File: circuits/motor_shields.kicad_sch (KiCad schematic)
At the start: 24 parts, among them IC1 BTN70301EPAXUMA1, IC2 BTN70301EPAXUMA1, IC3 BTN70301EPAXUMA1, IC4 BTN70301EPAXUMA1, J4 Conn_01x02_Pin, U2 74HC244

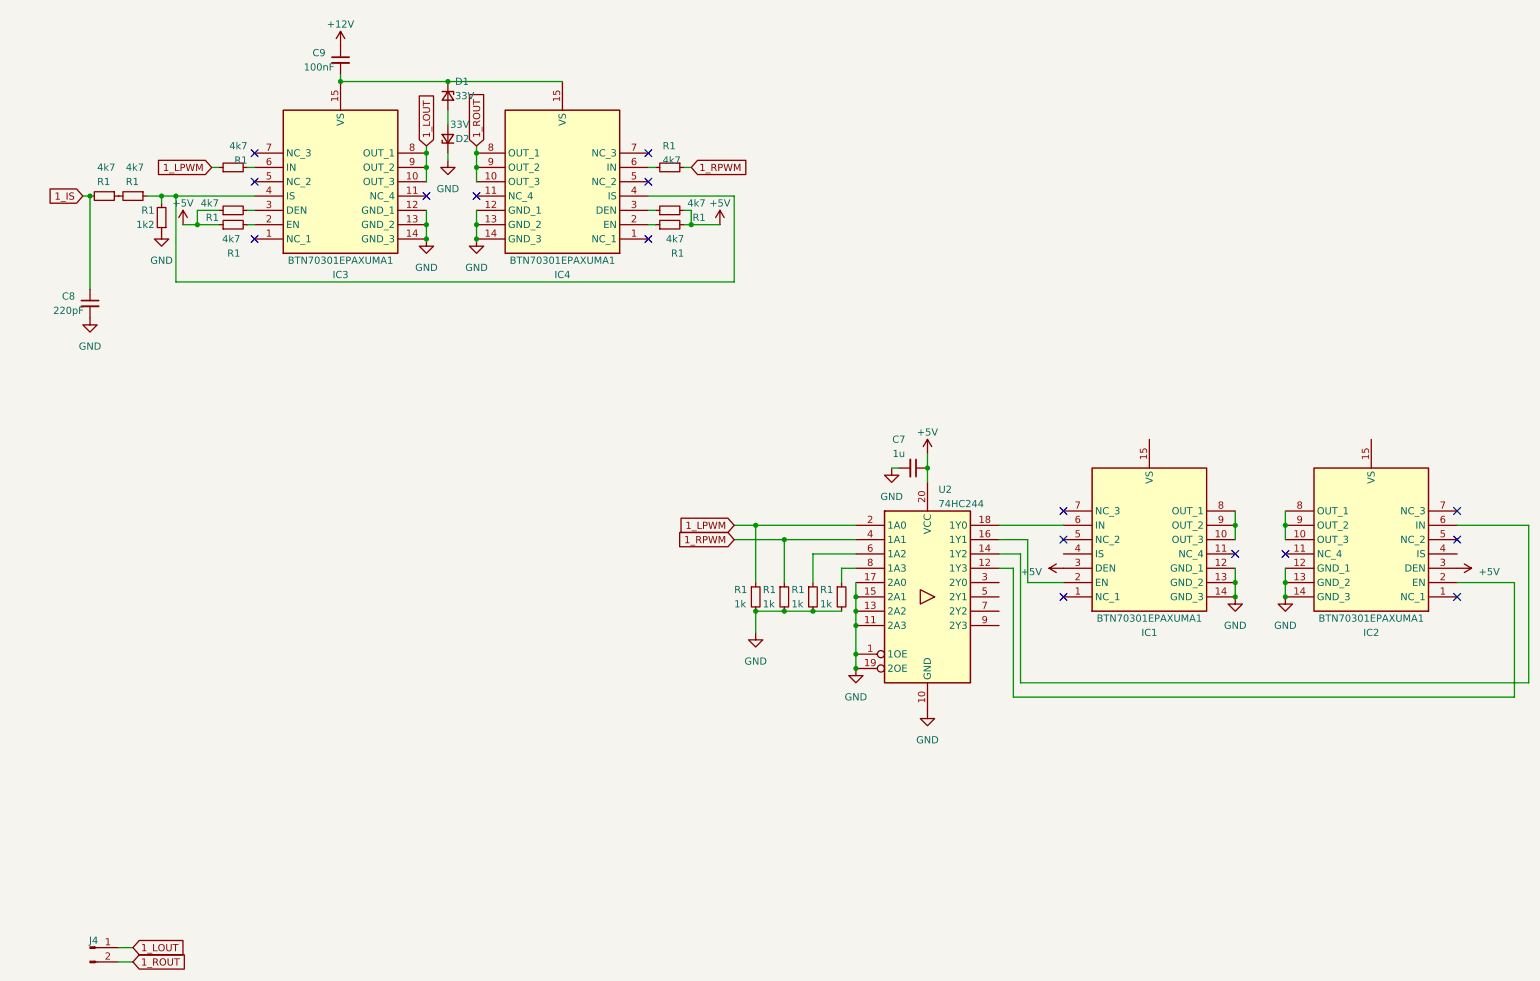
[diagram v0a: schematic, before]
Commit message: controller pcb rev 1
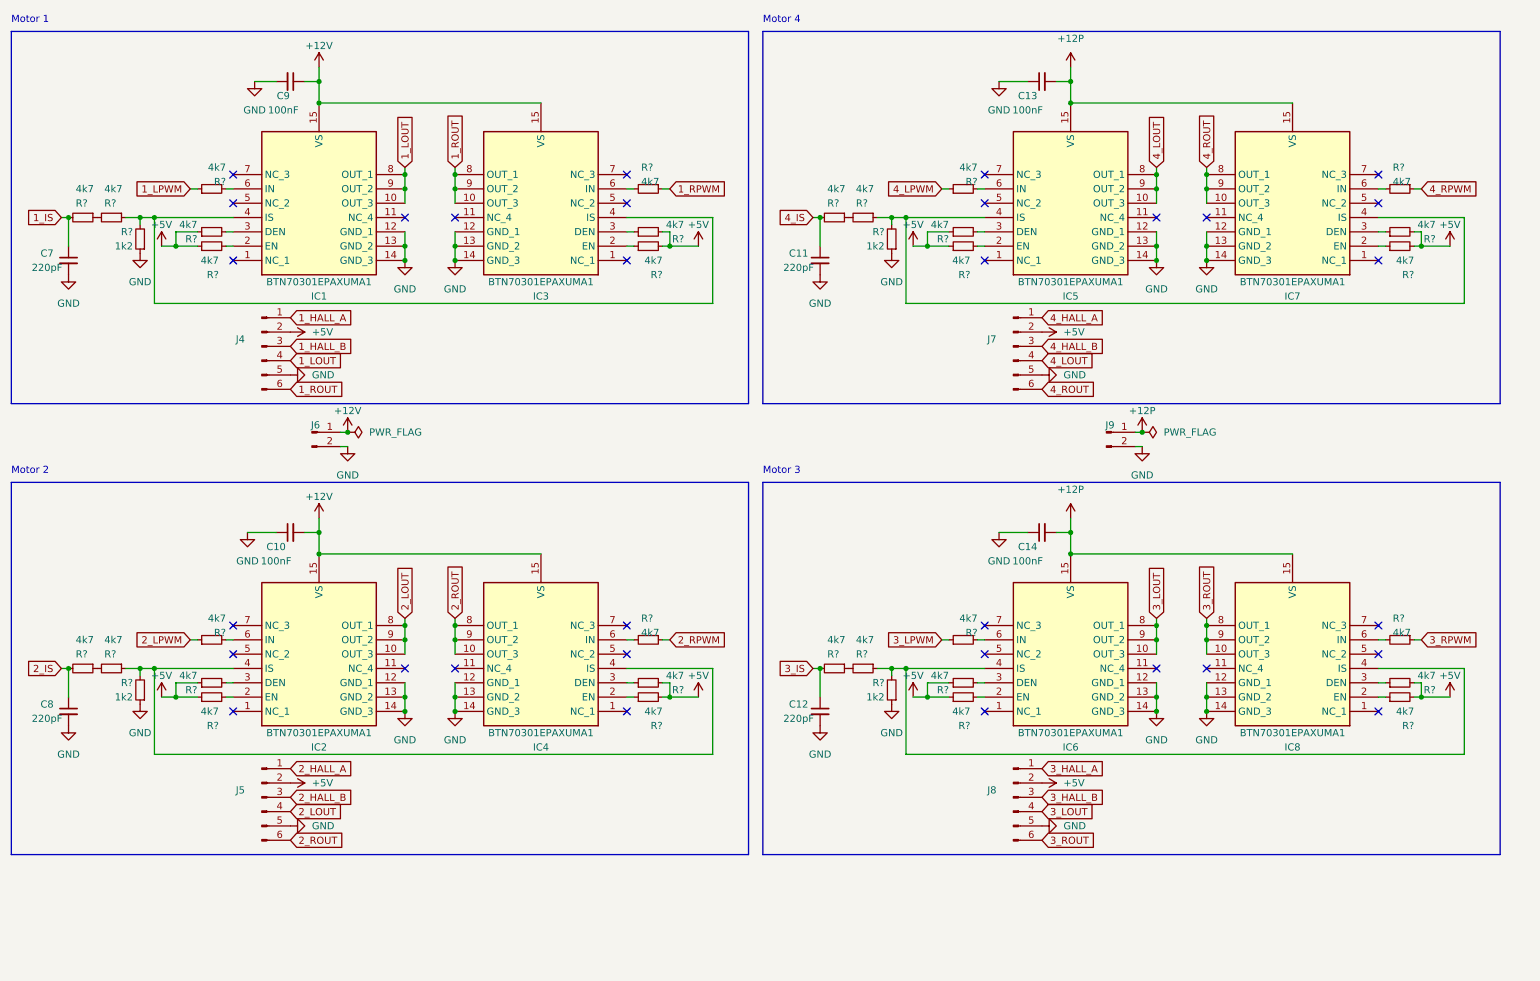
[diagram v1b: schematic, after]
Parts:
- removed C7: 1u, symbol Device:C_Small
- removed D1, D2: 33V, symbol Device:D_Zener_Small
- removed IC1: BTN70301EPAXUMA1, SOP65P600X115-15N, symbol SamacSys_Parts:BTN70301EPAXUMA1
- removed J4: Conn_01x02_Pin, symbol Connector:Conn_01x02_Pin
- removed R1 (x4): 1k, symbol Device:R_Small
- removed U2: 74HC244, symbol 74xx:74HC244
- added C10, C13, C14: 100nF, Capacitor_SMD:C_0603_1608Metric_Pad1.08x0.95mm_HandSolder, symbol Device:C_Small
- added C11, C12, C8: 220pF, Capacitor_SMD:C_0402_1005Metric_Pad0.74x0.62mm_HandSolder, symbol Device:C_Small
- added IC4, IC5, IC6, IC7, IC8: BTN70301EPAXUMA1, rbc Custom Library:Infineon_PG-TSDSO-14-22_custom, symbol SamacSys_Parts:BTN70301EPAXUMA1
- added J4, J5, J7, J8: Conn_01x06_Pin, Connector_Molex:Molex_Micro-Fit_3.0_43045-0612_2x03_P3.00mm_Vertical, symbol Connector:Conn_01x06_Pin
- added J6, J9: Conn_01x02_Pin, TerminalBlock_Phoenix:TerminalBlock_Phoenix_MKDS-3-2-5.08_1x02_P5.08mm_Horizontal, symbol Connector:Conn_01x02_Pin
- added R? (x24): 4k7, Resistor_SMD:R_1206_3216Metric_Pad1.30x1.75mm_HandSolder, symbol Device:R_Small
- added R? (x3): 1k2, Resistor_SMD:R_1206_3216Metric_Pad1.30x1.75mm_HandSolder, symbol Device:R_Small
- C7: renamed from C8; footprint (none) -> Capacitor_SMD:C_0402_1005Metric_Pad0.74x0.62mm_HandSolder
- C9: footprint (none) -> Capacitor_SMD:C_0603_1608Metric_Pad1.08x0.95mm_HandSolder
- IC1: renamed from IC3; footprint SOP65P600X115-15N -> rbc Custom Library:Infineon_PG-TSDSO-14-22_custom
- IC2: footprint SOP65P600X115-15N -> rbc Custom Library:Infineon_PG-TSDSO-14-22_custom
- IC3: renamed from IC4; footprint SOP65P600X115-15N -> rbc Custom Library:Infineon_PG-TSDSO-14-22_custom
- R? (x9): renamed from R1; footprint (none) -> Resistor_SMD:R_1206_3216Metric_Pad1.30x1.75mm_HandSolder
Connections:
- net +12V: now also IC1.15 (VS), IC2.15 (VS), IC3.15 (VS), C10.2, IC4.15 (VS), J6.1 (Pin_1)
- net +5V: now also J4.2 (Pin_2), J5.2 (Pin_2), J7.2 (Pin_2), J8.2 (Pin_2), R?.1, R?.1, R?.1, R?.1, R?.1, R?.1, R?.2, R?.2, R?.2, R?.2, R?.2, R?.2; no longer IC2.3 (DEN)
- net 1_LOUT: now also J4.4 (Pin_4)
- net 1_ROUT: now also J4.6 (Pin_6)
- net GND: now also C9.2, C10.1, C11.2, C12.2, C13.1, C14.1, C8.2, IC4.12 (GND_1), IC4.13 (GND_2), IC4.14 (GND_3), IC5.12 (GND_1), IC5.13 (GND_2), IC5.14 (GND_3), IC6.12 (GND_1), IC6.13 (GND_2), IC6.14 (GND_3), IC7.12 (GND_1), IC7.13 (GND_2), IC7.14 (GND_3), IC8.12 (GND_1), IC8.13 (GND_2), IC8.14 (GND_3), J4.5 (Pin_5), J5.5 (Pin_5), J6.2 (Pin_2), J7.5 (Pin_5), J8.5 (Pin_5), J9.2 (Pin_2), R?.1, R?.1, R?.1
- net at IC2.2 (EN): now also R?.2
- net at IC2.6 (IN): now also R?.2
- net 2_LOUT: now reaches IC2.10 (OUT_3), IC2.8 (OUT_1), IC2.9 (OUT_2)
- net 2_LOUT: now also J5.4 (Pin_4)
- net at IC2.4 (IS): now also IC4.4 (IS), R?.1, R?.2
- new net: R?.1, R?.2 (x3)
- new net: IC5.6 (IN), R?.2
- new net: IC8.2 (EN), R?.1
- new net: IC5.4 (IS), IC7.4 (IS), R?.1, R?.2
- new net: IC5.3 (DEN), R?.2
- new net: IC7.6 (IN), R?.2
- new net: IC6.4 (IS), IC8.4 (IS), R?.1, R?.2
- new net: IC4.6 (IN), R?.2
- new net: IC7.2 (EN), R?.1
- new net: IC7.3 (DEN), R?.1
- new net: IC8.6 (IN), R?.2
- new net: IC8.3 (DEN), R?.1
- new net: IC6.2 (EN), R?.2
- new net: IC6.3 (DEN), R?.2
- new net: IC6.6 (IN), R?.2
- new net: IC2.3 (DEN), R?.2
- new net: IC5.2 (EN), R?.2
- new net: IC4.2 (EN), R?.1
- new net: IC4.3 (DEN), R?.1
- new net +12P: C13.2, C14.2, IC5.15 (VS), IC6.15 (VS), IC7.15 (VS), IC8.15 (VS), J9.1 (Pin_1)
- new net 1_HALL_A: J4.1 (Pin_1)
- new net 1_HALL_B: J4.3 (Pin_3)
- new net 2_HALL_A: J5.1 (Pin_1)
- new net 2_HALL_B: J5.3 (Pin_3)
- new net 2_IS: C8.1, R?.2
- new net 2_LPWM: R?.1
- new net 2_ROUT: IC4.10 (OUT_3), IC4.8 (OUT_1), IC4.9 (OUT_2), J5.6 (Pin_6)
- new net 2_RPWM: R?.1
- new net 3_HALL_A: J8.1 (Pin_1)
- new net 3_HALL_B: J8.3 (Pin_3)
- new net 3_IS: C12.1, R?.2
- new net 3_LOUT: IC6.10 (OUT_3), IC6.8 (OUT_1), IC6.9 (OUT_2), J8.4 (Pin_4)
- new net 3_LPWM: R?.1
- new net 3_ROUT: IC8.10 (OUT_3), IC8.8 (OUT_1), IC8.9 (OUT_2), J8.6 (Pin_6)
- new net 3_RPWM: R?.1
- new net 4_HALL_A: J7.1 (Pin_1)
- new net 4_HALL_B: J7.3 (Pin_3)
- new net 4_IS: C11.1, R?.2
- new net 4_LOUT: IC5.10 (OUT_3), IC5.8 (OUT_1), IC5.9 (OUT_2), J7.4 (Pin_4)
- new net 4_LPWM: R?.1
- new net 4_ROUT: IC7.10 (OUT_3), IC7.8 (OUT_1), IC7.9 (OUT_2), J7.6 (Pin_6)
- new net 4_RPWM: R?.1
- no-connect marks 16 -> 32
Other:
- note added: "Motor 1"
- note added: "Motor 2"
- note added: "Motor 3"
- note added: "Motor 4"
- moved on the sheet: C7, C9, IC1, IC3, R?
